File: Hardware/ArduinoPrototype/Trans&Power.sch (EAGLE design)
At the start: 20 parts, among them U1 MCP2551, U4 MCP2551, U5 TLF1963TBATMA1

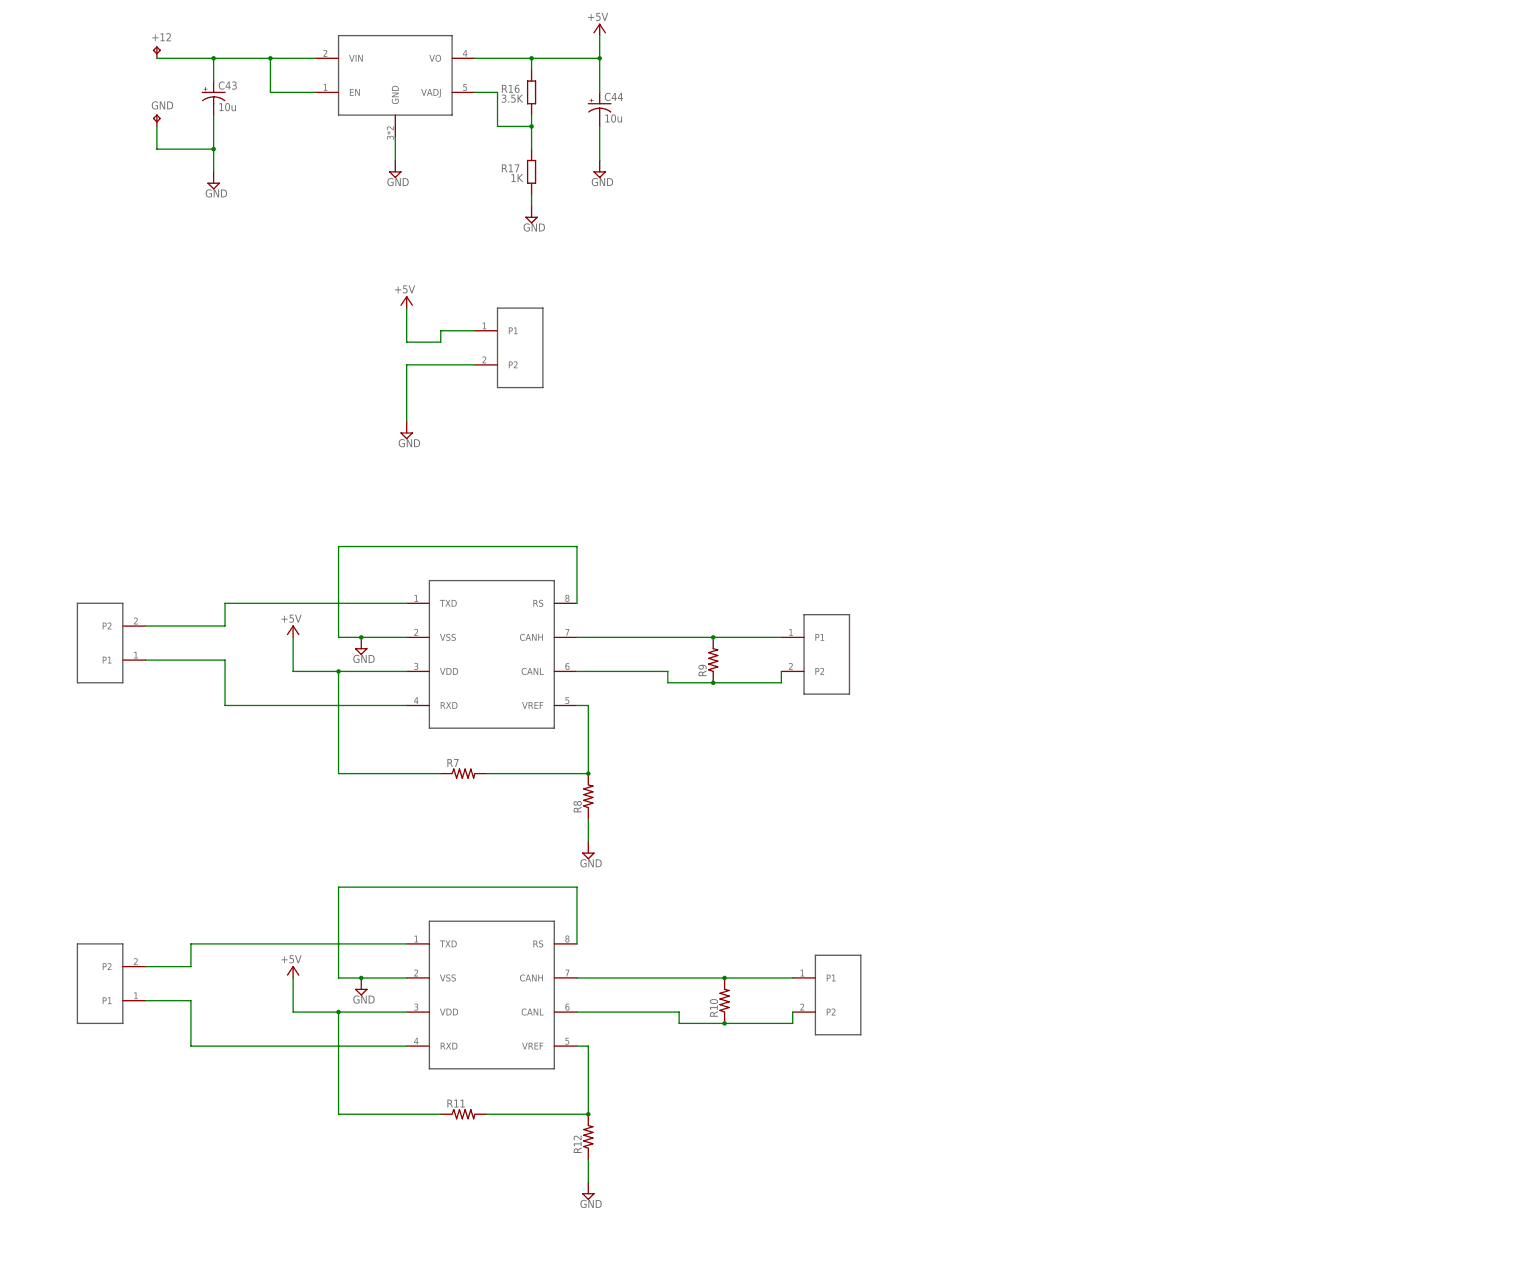
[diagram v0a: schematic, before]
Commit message: jaime
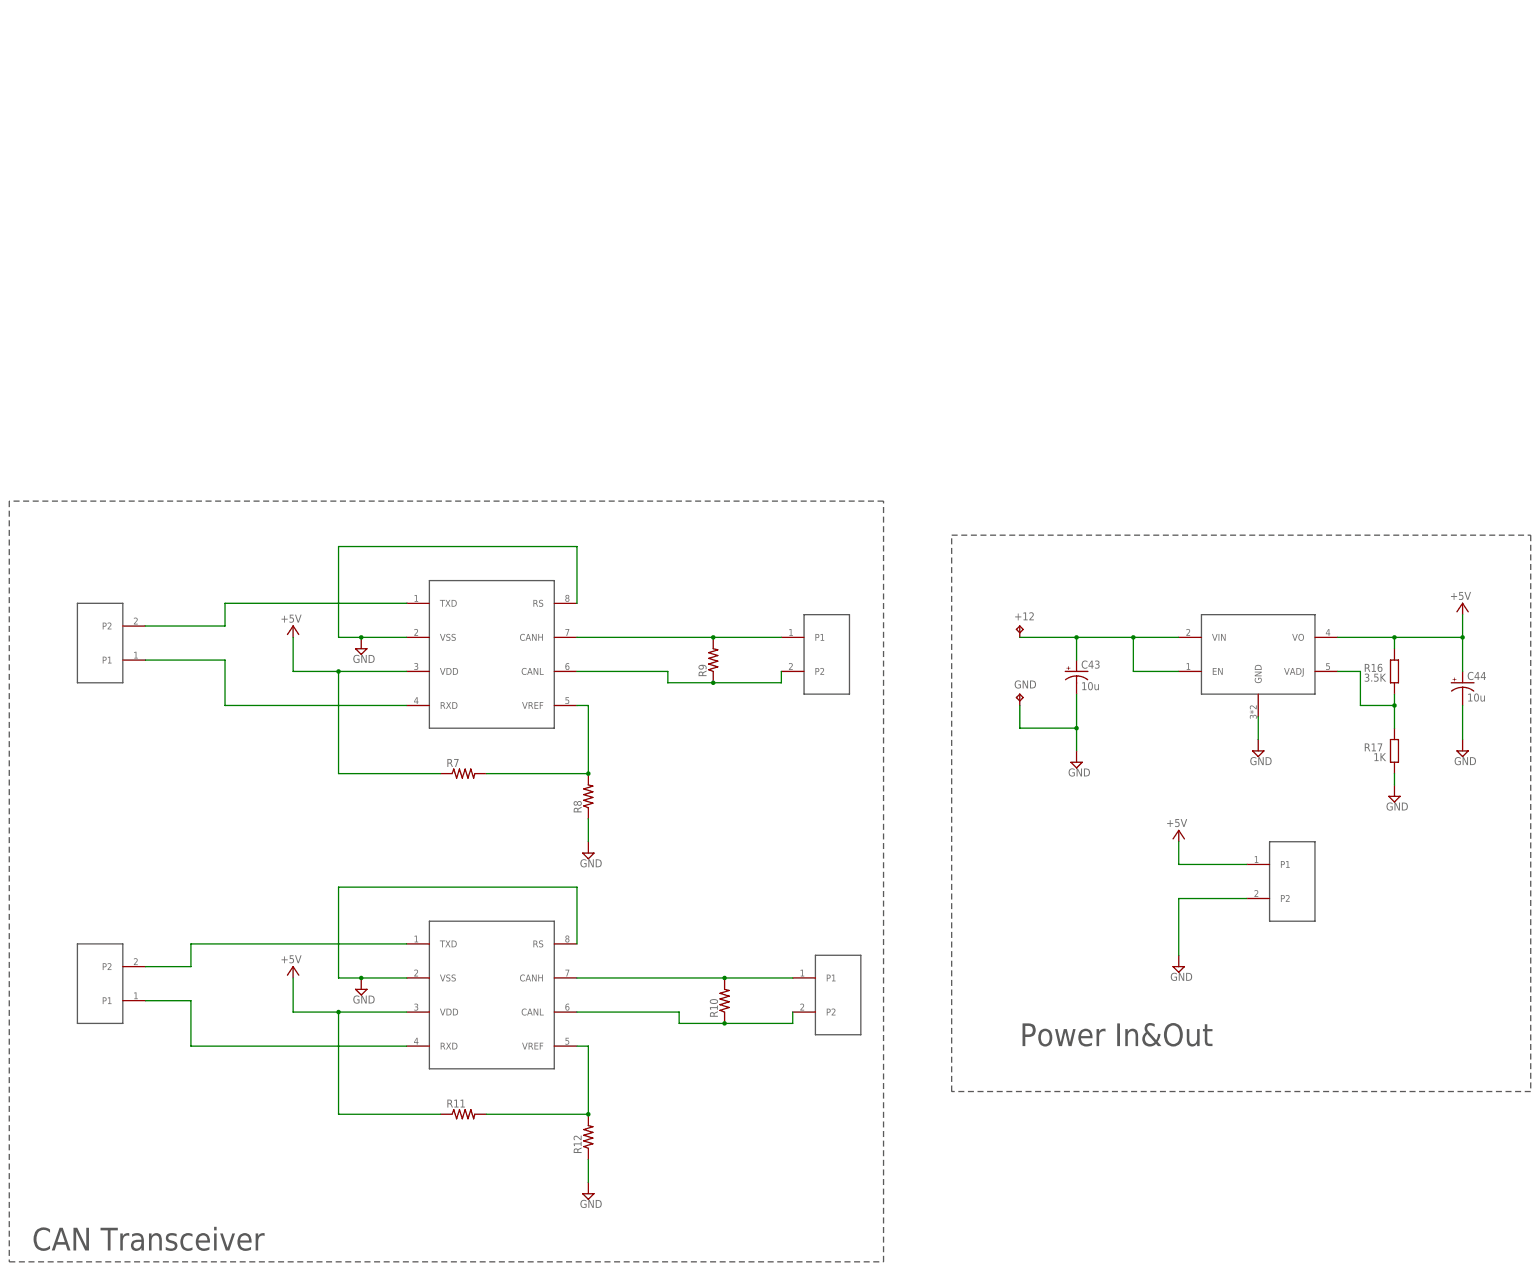
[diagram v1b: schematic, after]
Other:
- note added: "CAN Transceiver"
- note added: "Power In&Out"
- moved on the sheet: +12, C43, C44, GND, R16, R17
